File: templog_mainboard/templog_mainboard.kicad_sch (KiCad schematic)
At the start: 3 parts, among them U1 ESP32-S3-MINI-1, U2 DS3231MZ, U3 SHT4x

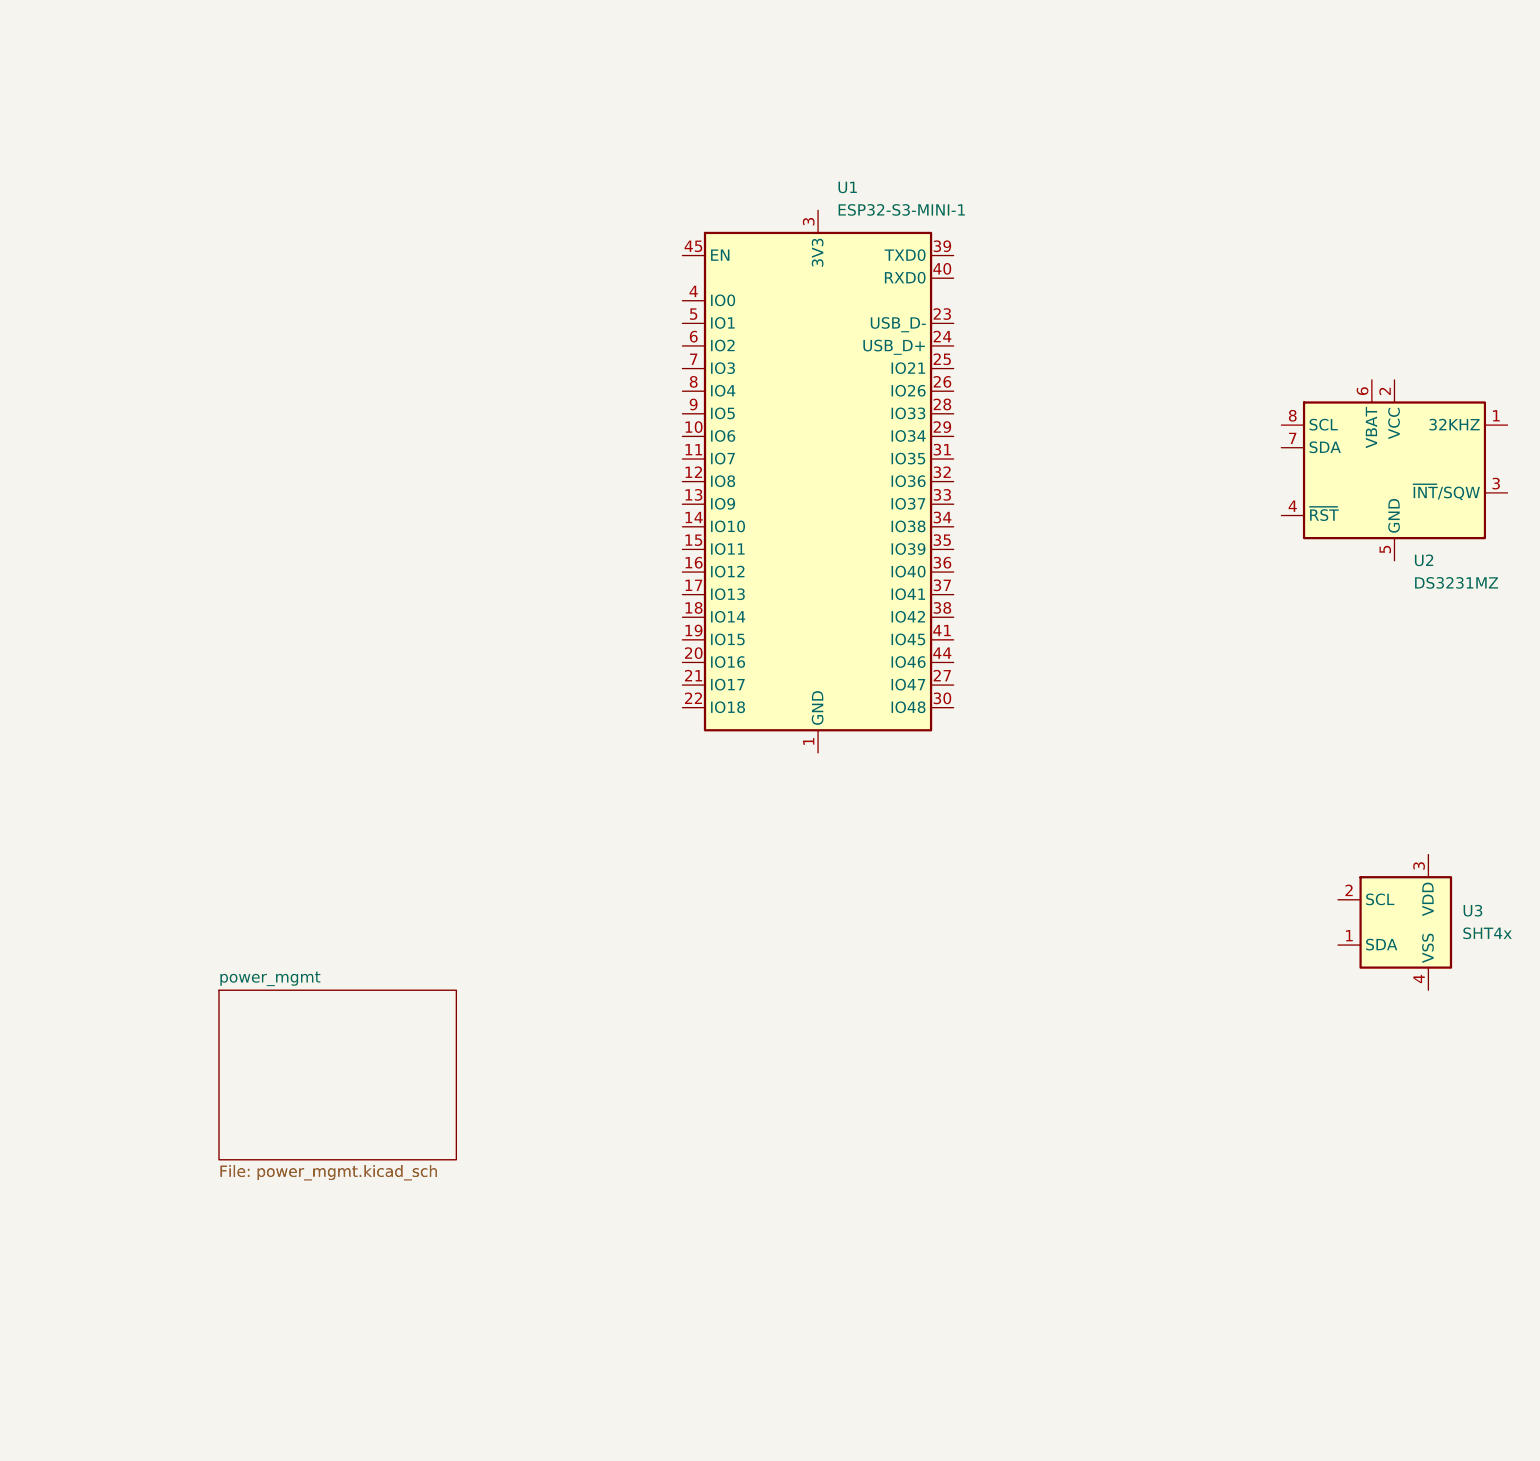
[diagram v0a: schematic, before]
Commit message: elecricity
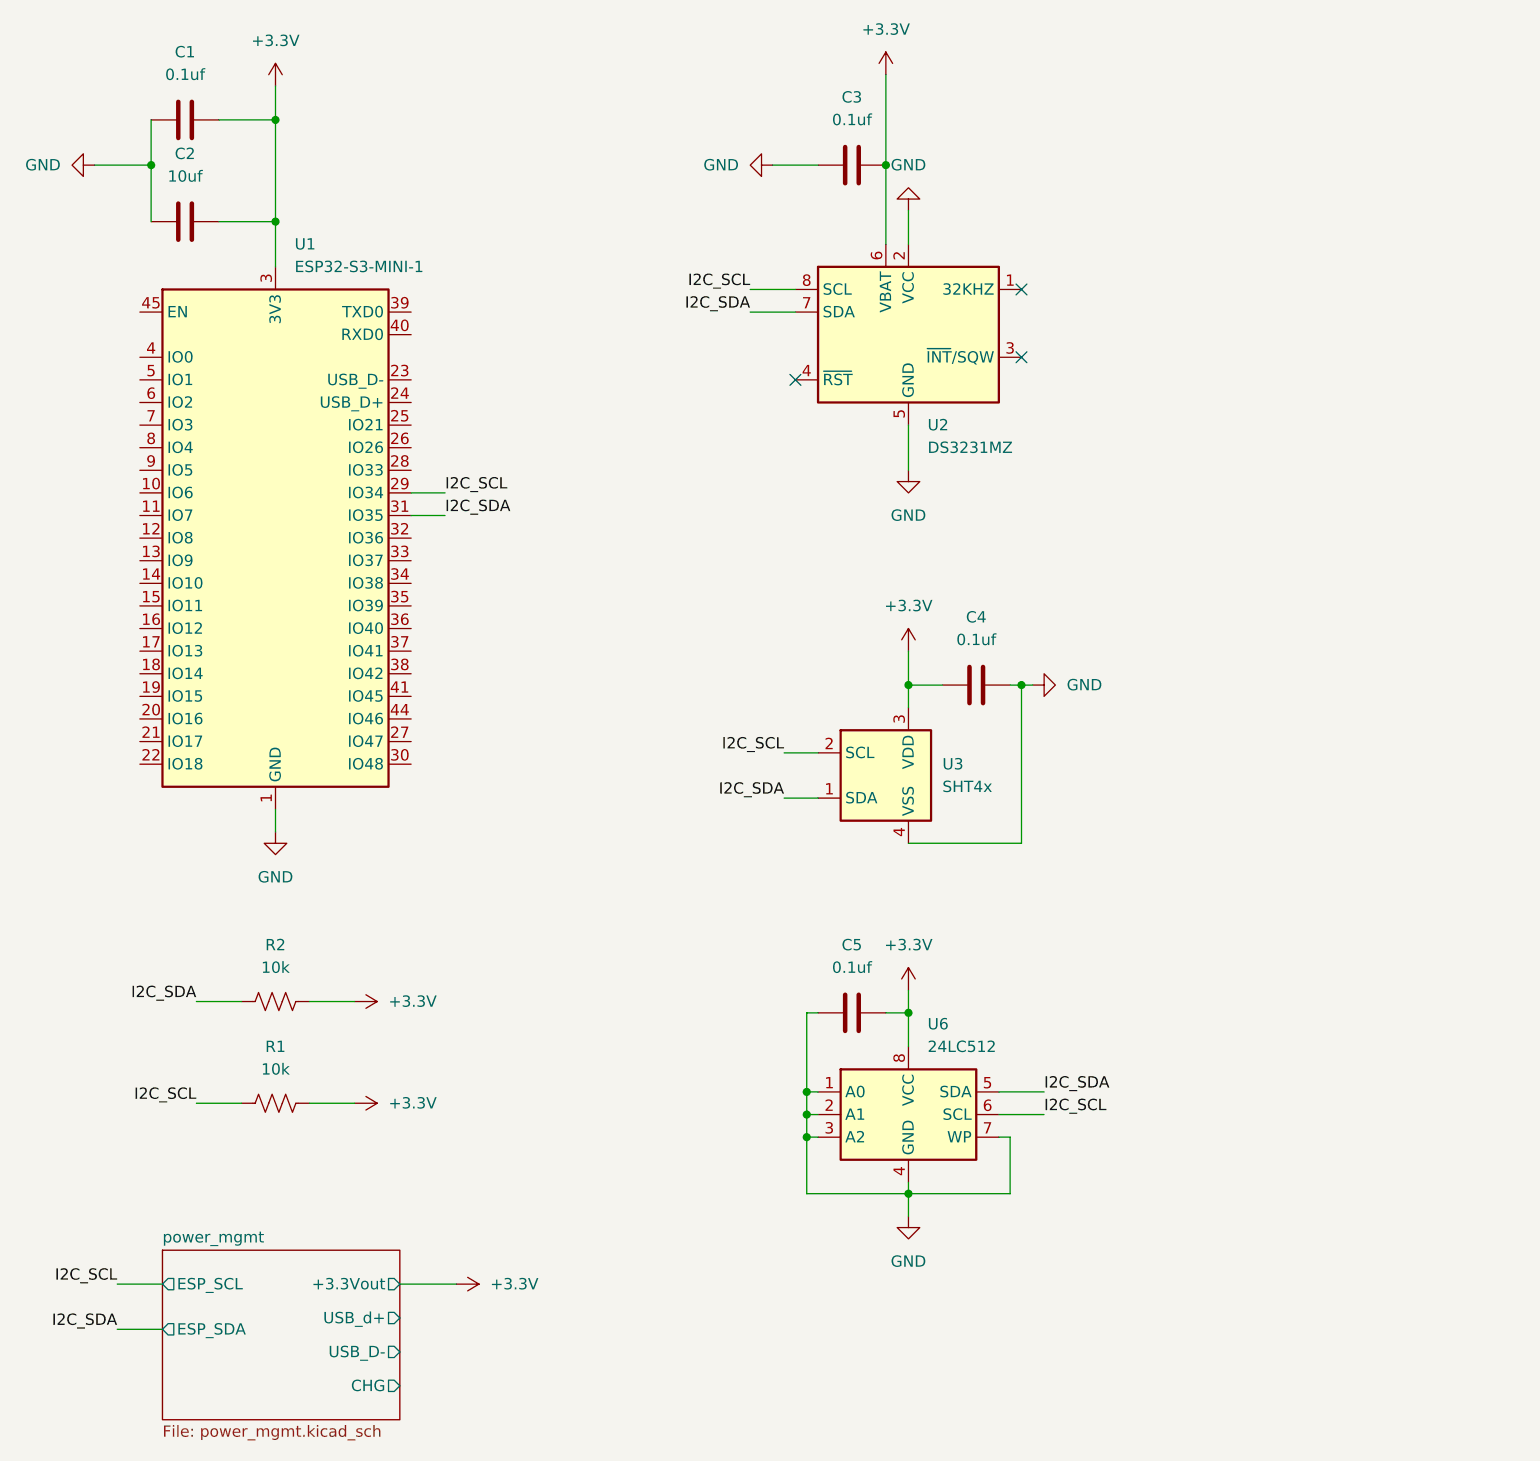
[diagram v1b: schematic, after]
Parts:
- added C1, C3, C4, C5: 0.1uf, Capacitor_SMD:C_0201_0603Metric, symbol Device:C
- added C2: 10uf, Capacitor_SMD:C_0201_0603Metric, symbol Device:C
- added R1, R2: 10k, symbol Device:R_US
- added U6: 24LC512, symbol Memory_EEPROM:24LC512
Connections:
- net I2C_SDA: now reaches U3.1 (SDA)
- net I2C_SDA: now also U1.31 (IO35), U2.7 (SDA), R2.1, U6.5 (SDA)
- net I2C_SCL: now reaches U3.2 (SCL)
- net I2C_SCL: now also U1.29 (IO34), U2.8 (SCL), R1.1, U6.6 (SCL)
- net +3.3V: now reaches U3.3 (VDD)
- net +3.3V: now also U1.3 (3V3), U2.6 (VBAT), C1.2, C2.2, C3.2, C4.1, C5.2, R1.2, R2.2, U6.8 (VCC)
- net GND: now reaches U3.4 (VSS)
- net GND: now also U1.1 (GND), U1.2 (GND), U1.42 (GND), U1.43 (GND), U1.46 (GND), U1.47 (GND), U1.48 (GND), U1.49 (GND), U1.50 (GND), U1.51 (GND), U1.52 (GND), U1.53 (GND), U1.54 (GND), U1.55 (GND), U1.56 (GND), U1.57 (GND), U1.58 (GND), U1.59 (GND), U1.60 (GND), U1.61 (GND), U1.62 (GND), U1.63 (GND), U1.64 (GND), U1.65 (GND), U2.2 (VCC), U2.5 (GND), C1.1, C2.1, C3.1, C4.2, C5.1, U6.1 (A0), U6.2 (A1), U6.3 (A2), U6.4 (GND), U6.7 (WP)
- no-connect marks 0 -> 3
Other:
- sheet power_mgmt ports: added +3.3Vout, CHG, ESP_SCL, ESP_SDA, USB_D-, USB_d+; removed none
- moved on the sheet: U1, U2, U3
